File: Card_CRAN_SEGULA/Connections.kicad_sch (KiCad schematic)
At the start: 34 parts, among them J1 503398-1892, J2 USB4110GFA, J3 USB4110GFA, J6 M50-3600542R, J7 M50-3600542R

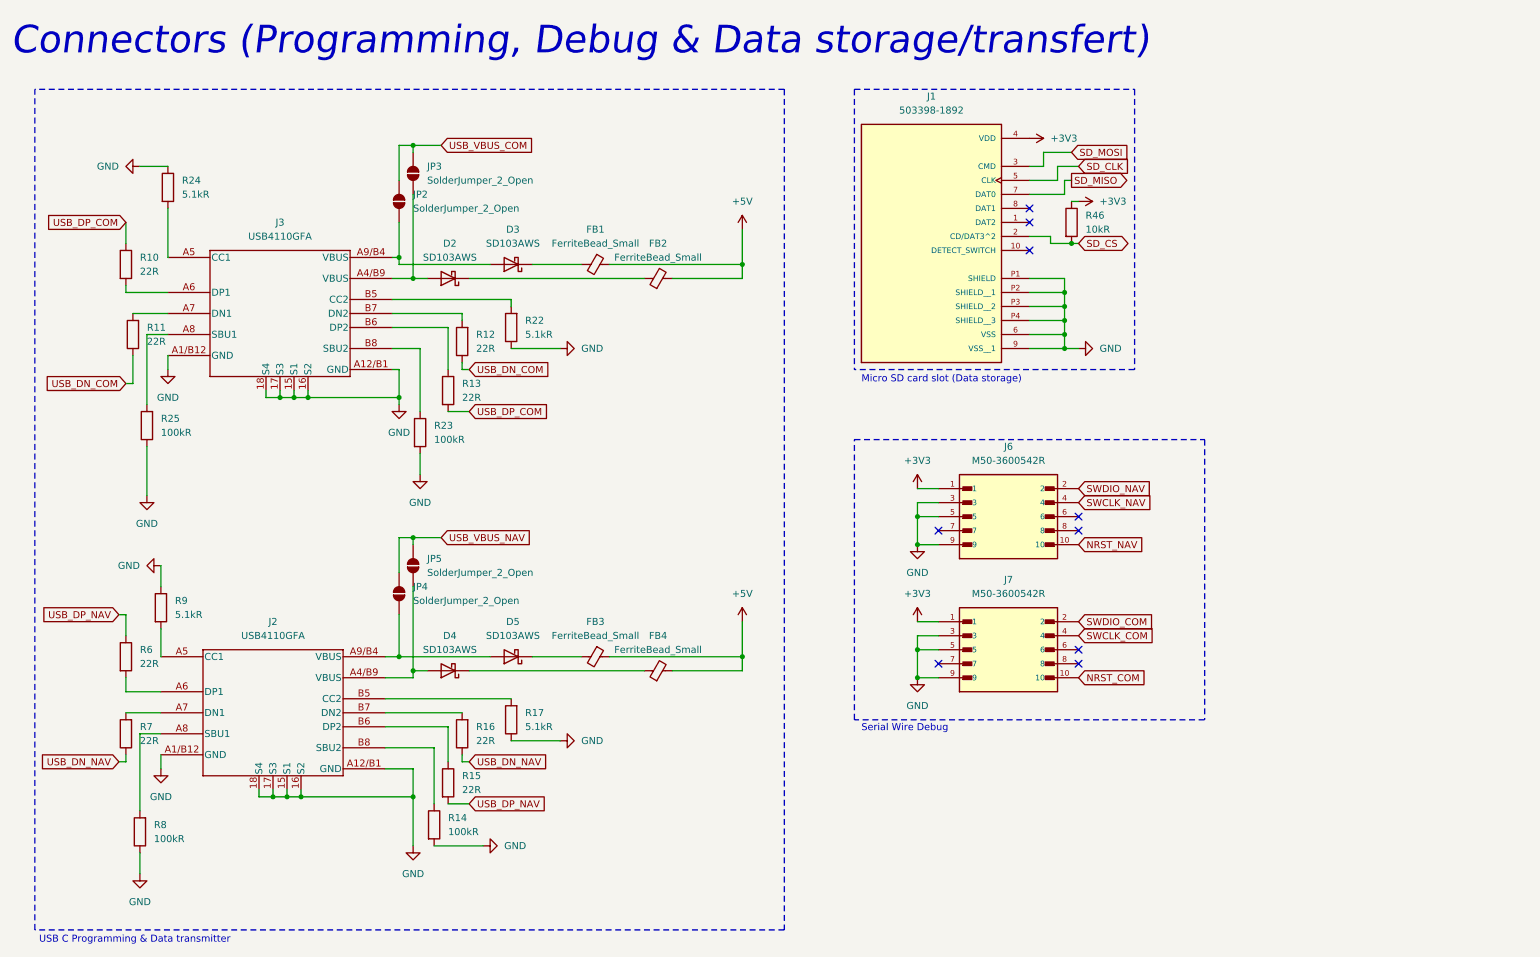
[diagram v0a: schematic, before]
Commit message: MàJ 07/07/2025
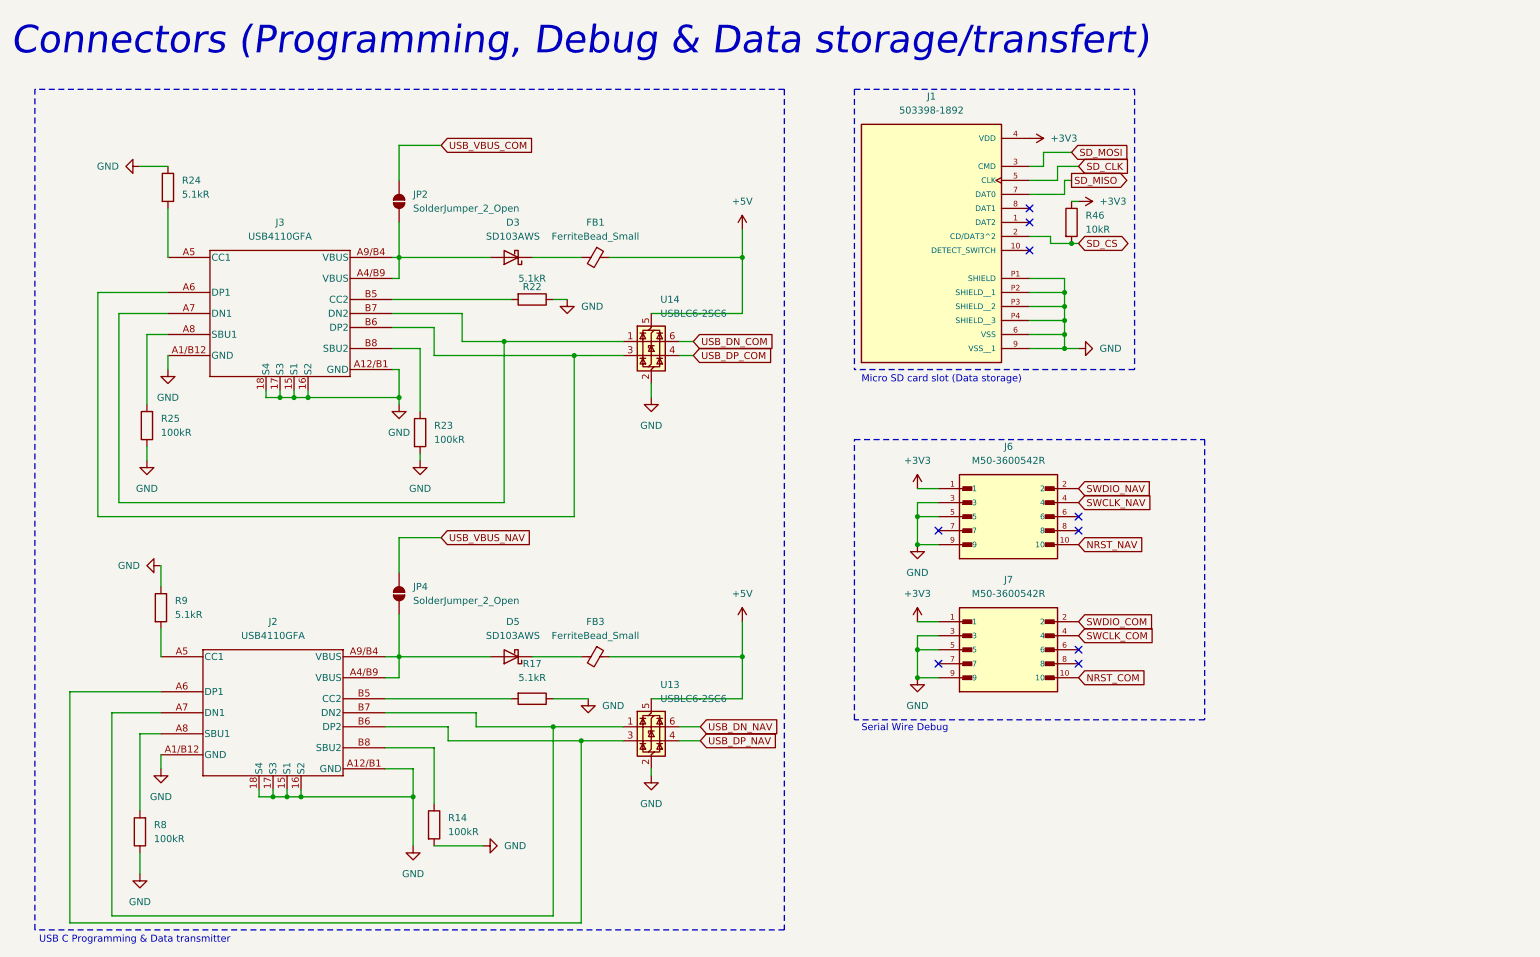
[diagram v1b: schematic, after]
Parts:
- removed D2, D4: SD103AWS, D_Schottky_SD103AWS:D_SOD-323, symbol schottky_SD103AWS:D_Schottky
- removed FB2, FB4: FerriteBead_Small, FERRITE_BEAD_120_OHM_0402_4LN_MPZ1005S121HT000:L_0402_1005Metric, symbol ferritebead_small:FerriteBead_Small
- removed JP3, JP5: SolderJumper_2_Open, SolderJumper_2_Open:SolderJumper-2_P1.3mm_Open_RoundedPad1.0x1.5mm, symbol solderjumper_2_open:SolderJumper_2_Open
- removed R10, R11, R12, R13, R15, R16, R6, R7: 22R, Resistor_22R_ERA-2AKD220X:RES_ERA2AKD220X, symbol Resistor:R
- added U13, U14: USBLC6-2SC6, Package_TO_SOT_SMD:SOT-23-6, symbol Power_Protection:USBLC6-2SC6
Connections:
- net +5V: now also U13.5 (VBUS), U14.5 (VBUS)
- net GND: now also U13.2 (GND), U14.2 (GND)
- net USB_DN_COM: now also U14.6 (I/O1)
- net USB_DN_NAV: now also U13.6 (I/O1)
- net USB_DP_COM: now also U14.4 (I/O2)
- net USB_DP_NAV: now also U13.4 (I/O2)
- net at D3.2 (A), J3.A9/B4 (VBUS), JP2.1 (A): now also J3.A4/B9 (VBUS)
- net at J2.B7 (DN2): now also J2.A7 (DN1), U13.1 (I/O1)
- net at J3.B7 (DN2): now also J3.A7 (DN1), U14.1 (I/O1)
- net at D5.2 (A), J2.A9/B4 (VBUS), JP4.1 (A): now also J2.A4/B9 (VBUS)
- net at J3.A6 (DP1): now also J3.B6 (DP2), U14.3 (I/O2)
- net at J2.A6 (DP1): now also J2.B6 (DP2), U13.3 (I/O2)
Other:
- moved on the sheet: D3, FB1, R17, R22
